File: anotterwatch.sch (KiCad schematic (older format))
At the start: 26 parts, among them J1 USB_C_Receptacle_USB2.0, Q1 Q_NMOS_GSD, U1 USBLC6-4SC6

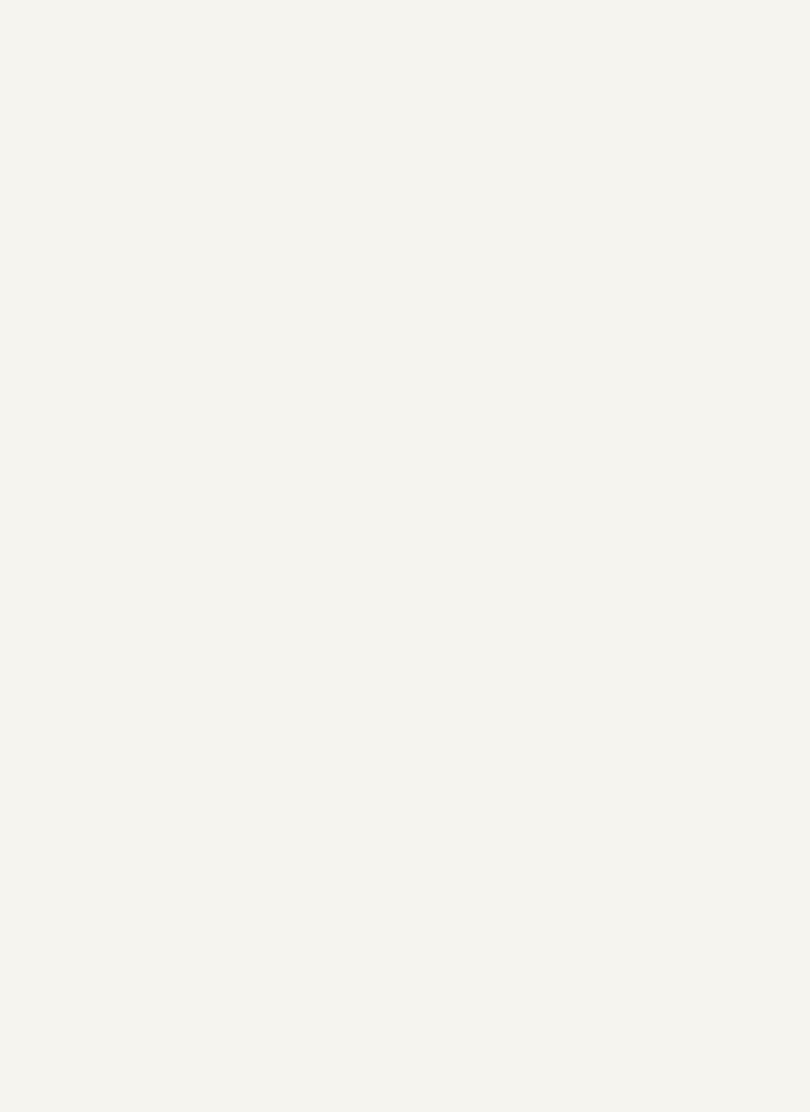
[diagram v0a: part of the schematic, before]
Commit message: added esp
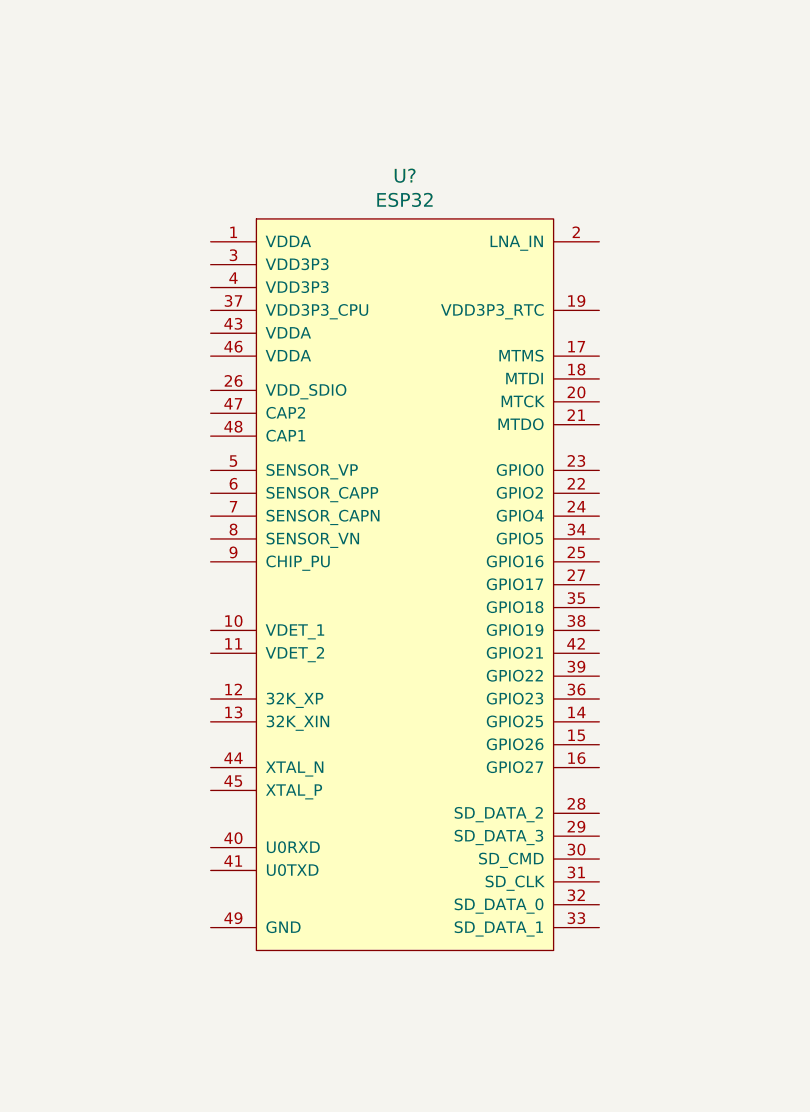
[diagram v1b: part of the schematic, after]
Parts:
- added U?: ESP32, ESP32-footprints-Lib:ESP32, symbol ESP32-footprints-Shem-Lib:ESP32
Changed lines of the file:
@@
 Text GLabel 10950 3800 1    50   Input ~ 0
 EN
+$Comp
+L ESP32-footprints-Shem-Lib:ESP32 U?
+U 1 1 5C71E383
+P 5050 3500
+F 0 "U?" H 5050 5337 60  0000 C CNN
+F 1 "ESP32" H 5050 5231 60  0000 C CNN
+F 2 "ESP32-footprints-Lib:ESP32" H 5050 1875 60  0001 C CNN
+F 3 "https://www.espressif.com/sites/default/files/documentation/esp32-pico-d4_datasheet_en.pdf" H 5500 4400 60  0001 C CNN
+F 4 "https://github.com/adamjvr/ESP32-kiCAD-Footprints" H 5050 3500 50  0001 C CNN "Lib"
+	1    5050 3500
+	1    0    0    -1
+$EndComp
 $EndSCHEMATC
